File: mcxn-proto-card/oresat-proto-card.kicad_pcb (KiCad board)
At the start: 4 copper layers, 99.8 x 94.6 mm, 141 parts, among them J1 J-SAMTEC-TFM-120-X1-XXX-D-RA, J10 61083-061409LF, J11 436500201, J14 ESQ-126-12-G-D, J15 ESQ-126-12-G-D, J3 SM14B-SHLS-TF, Q1 DMP2240UDM, Q2 DMP3050LVT-7, Q7 DMP3050LVT-7, Q8 PMV45EN, Q9 PMV45EN, U1 MCXN947VKLT, U10 TPS62111RSA, U11 MIC842LYC5, U12 MIC842LYC5, U2 MAX7310, U3 TS5A21366DCUR, U6 MAX4211FETE, U8 TCAN330, Y2 24 MHz

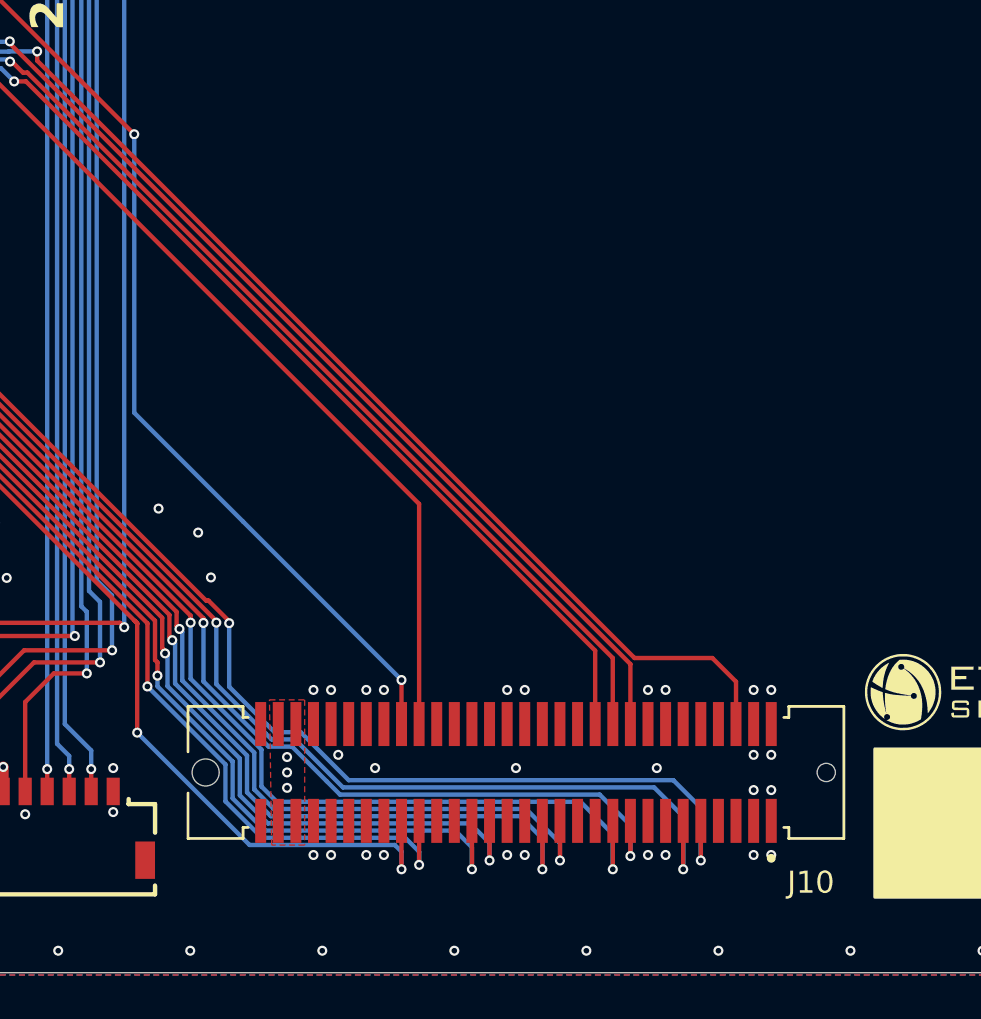
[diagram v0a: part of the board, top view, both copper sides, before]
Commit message: Adjusted RF connection
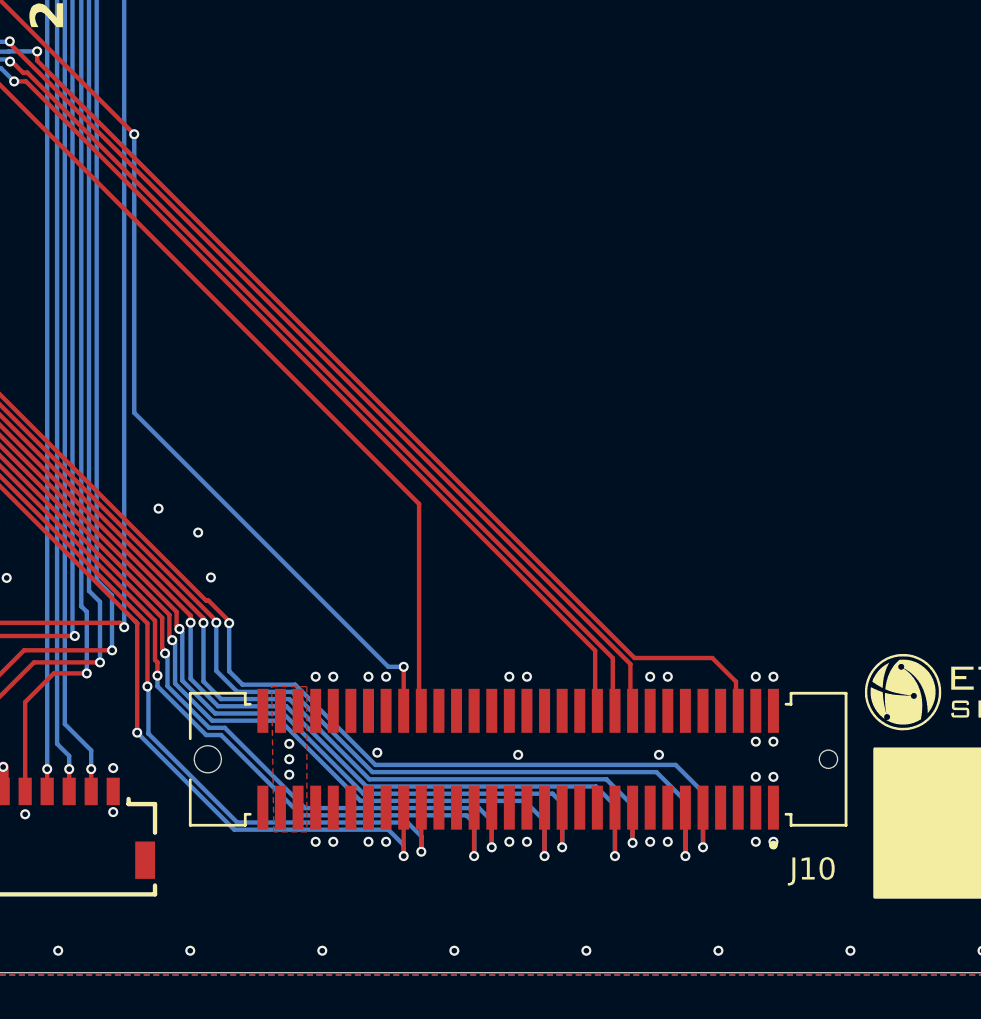
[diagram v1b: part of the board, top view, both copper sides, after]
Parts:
- moved J10 0.61 mm to (148.5, 142.6)
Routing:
- net /Microcontroller/P3_13: track 85.7 -> 84.7 mm
- net /Microcontroller/P3_14: track 84.4 -> 83.5 mm
- net /Microcontroller/P3_15: track 90.9 -> 90.1 mm
- net /Microcontroller/P3_11: track 89.4 -> 88.7 mm
- net /Microcontroller/P3_8: track 89.7 -> 89.1 mm
- net GND: vias 261 -> 260
